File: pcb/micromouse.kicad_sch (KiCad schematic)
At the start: 13 parts, among them U1 TSSP77038ETR, U2 TSSP77038ETR, U3 TSSP77038ETR, U4 TSSP77038ETR, U5 TSSP77038ETR, U6 TSSP77038ETR, U7 ATmega328PB-A, Y1 Crystal

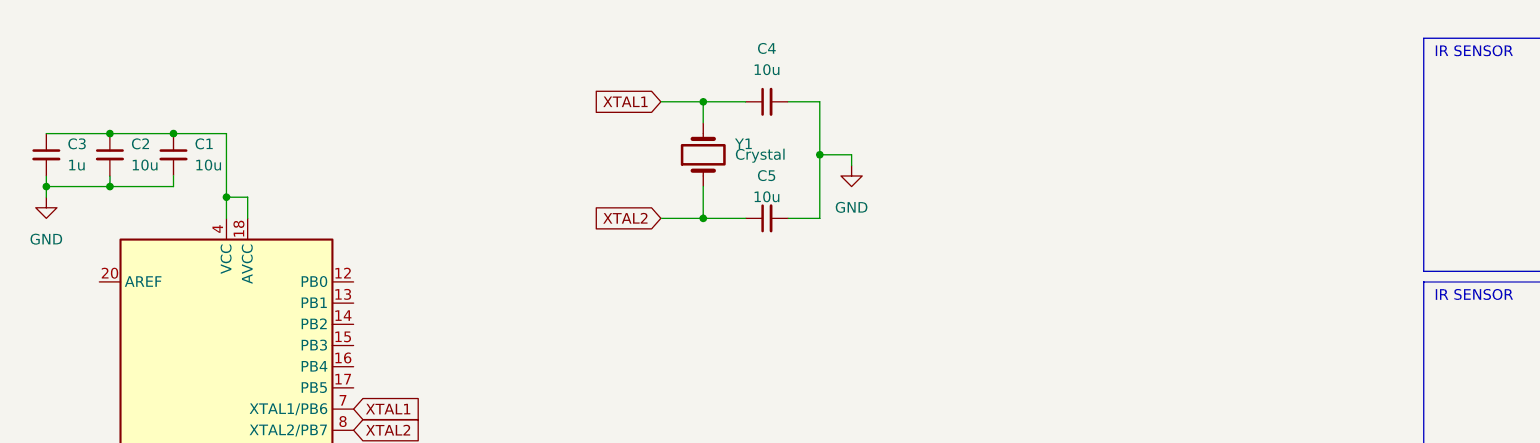
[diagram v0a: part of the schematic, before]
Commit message: add program port
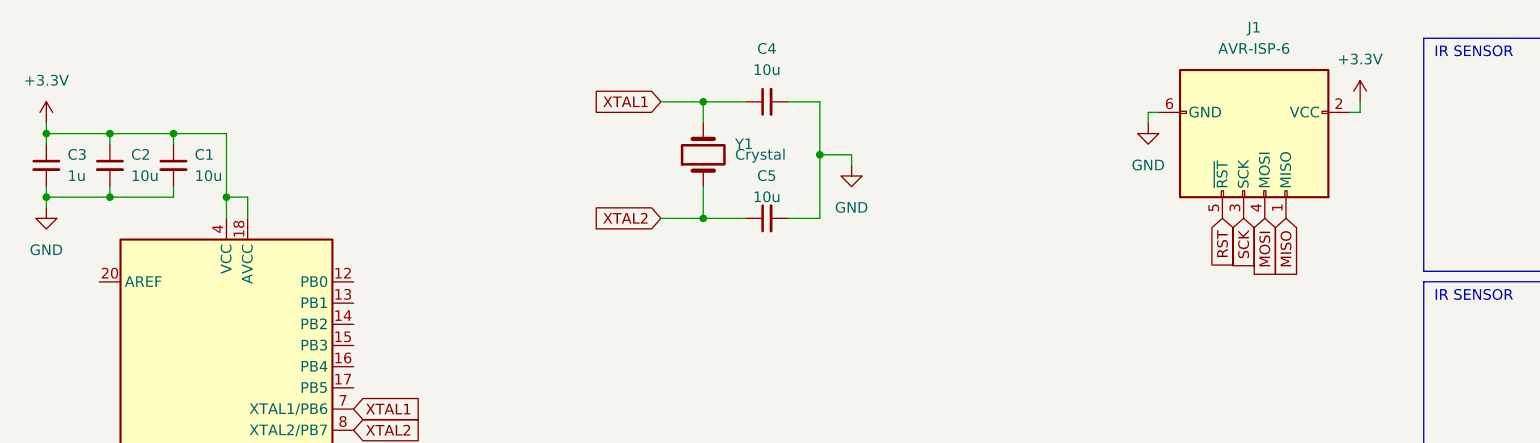
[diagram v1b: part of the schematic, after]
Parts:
- added J1: AVR-ISP-6, symbol Connector:AVR-ISP-6
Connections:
- net +3.3V: now also C1.1, C2.1, C3.1, U7.18 (AVCC), U7.4 (VCC), J1.2 (VCC)
- net GND: now also J1.6 (GND)
- new net MISO: J1.1 (MISO)
- new net MOSI: J1.4 (MOSI)
- new net RST: J1.5 (~{RST})
- new net SCK: J1.3 (SCK)
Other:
- moved on the sheet: C1, C2, C3
